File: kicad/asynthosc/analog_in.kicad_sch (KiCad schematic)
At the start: 18 parts, among them J2 AudioJack2, J5 AudioJack2, Q1 Q_NPN_BEC, SW1 TRG0, SW2 ${SIM.PARAMS}, U3 MCP6004

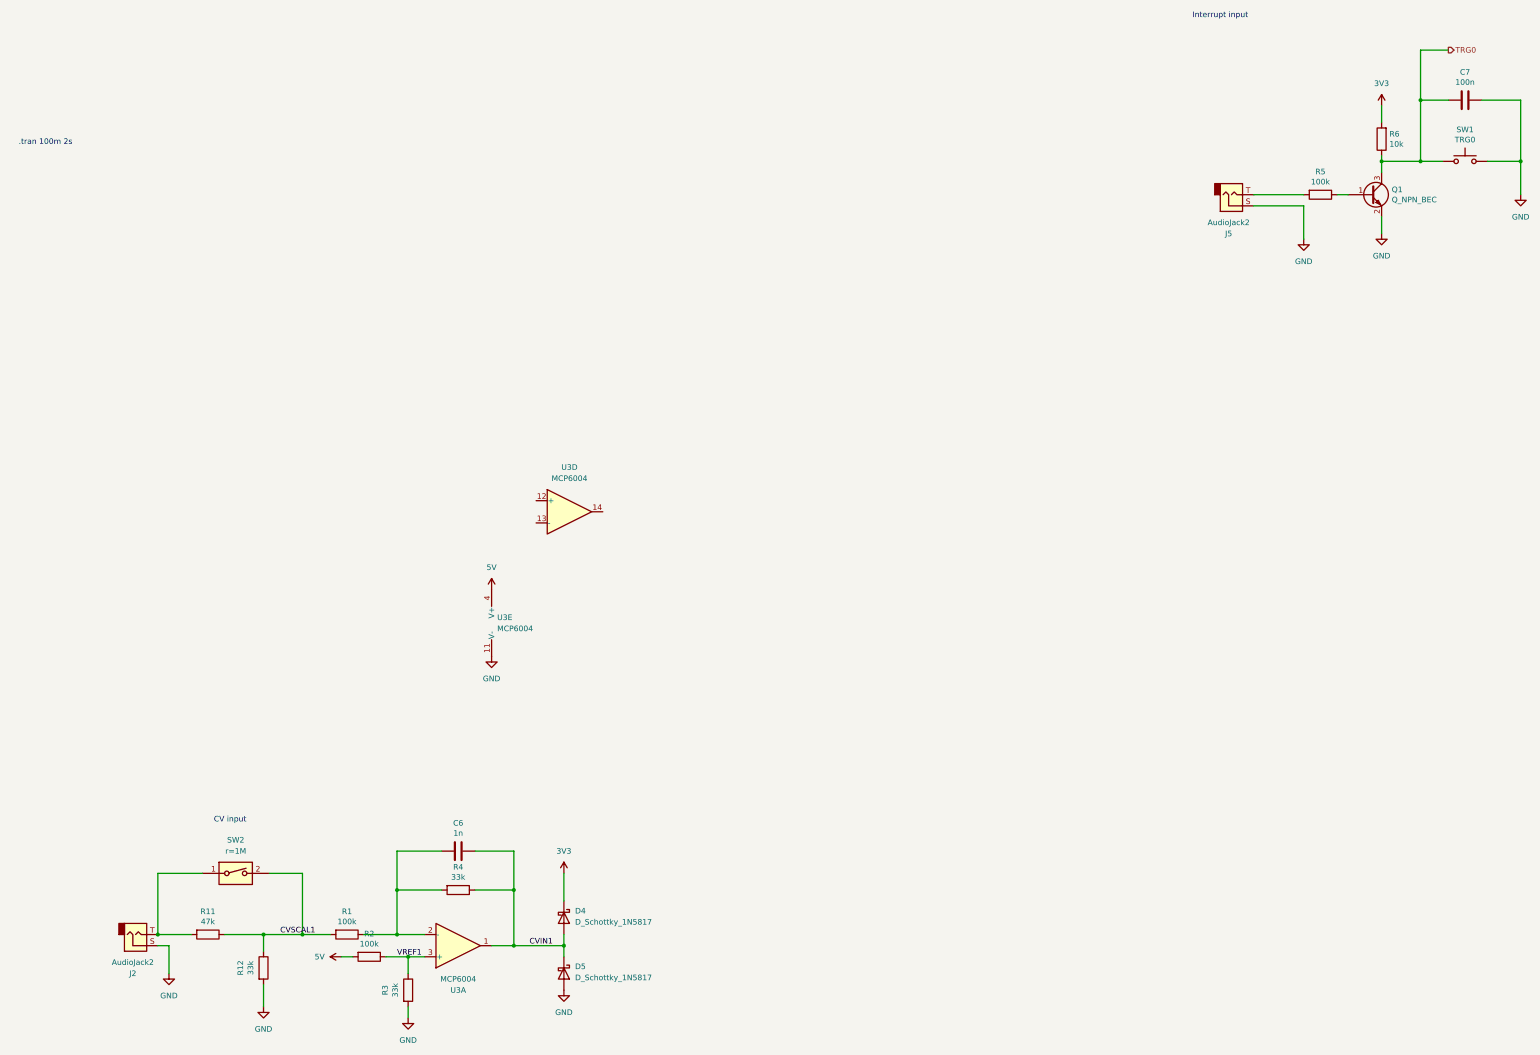
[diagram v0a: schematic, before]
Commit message: sch: wip
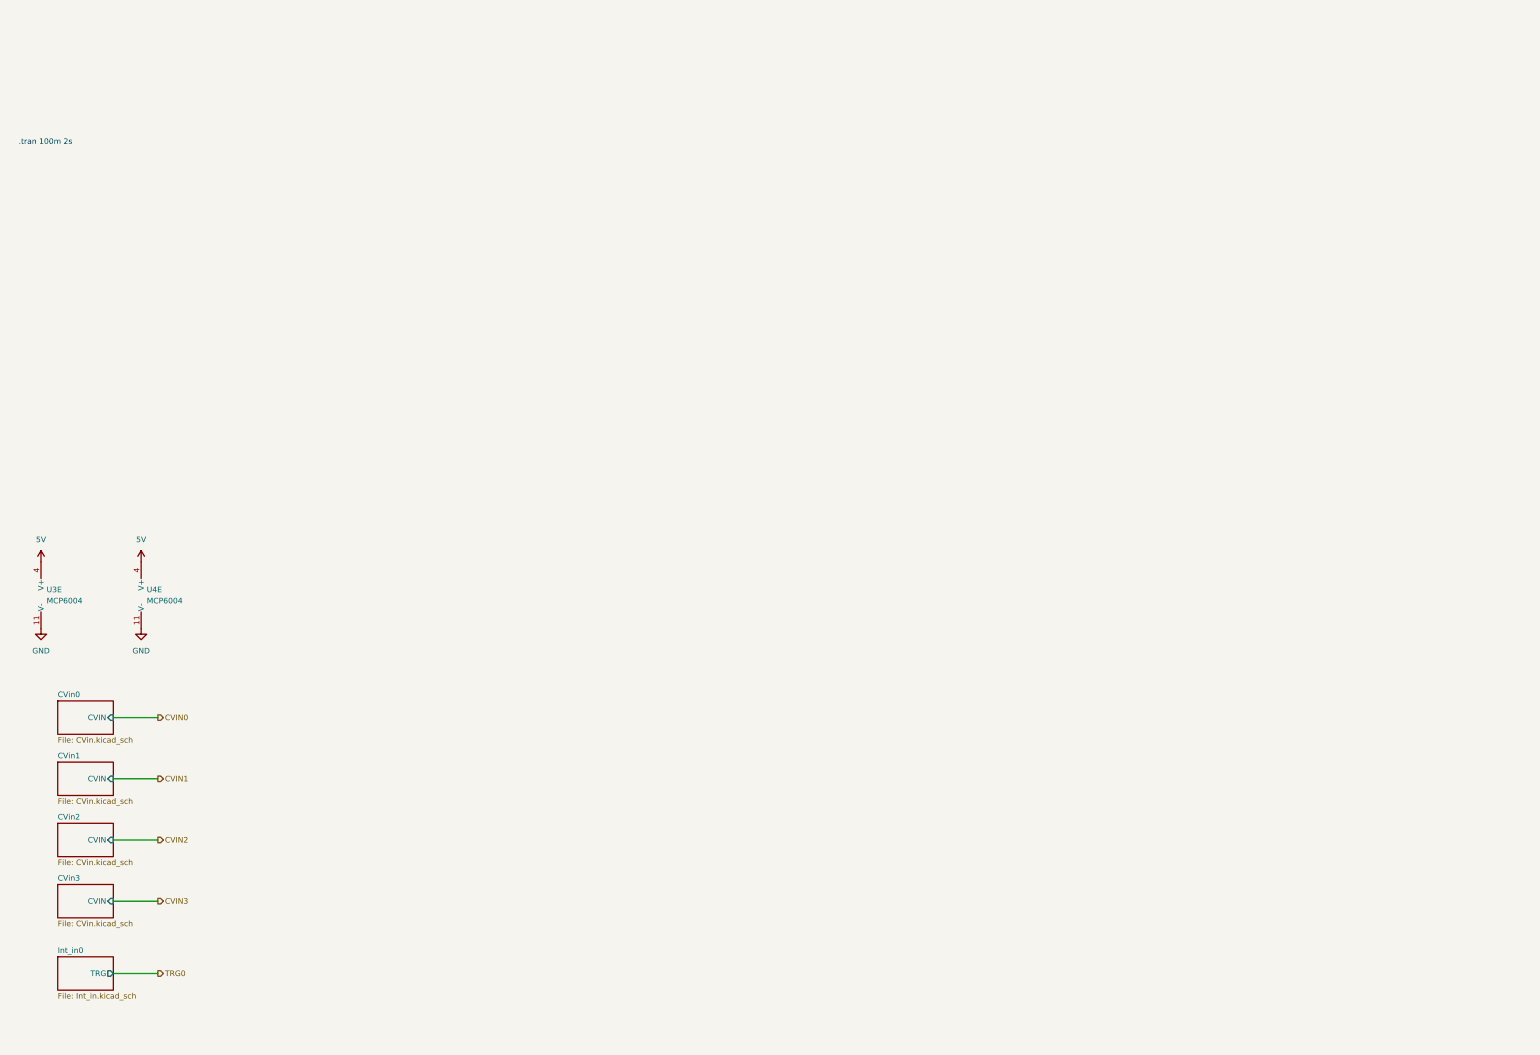
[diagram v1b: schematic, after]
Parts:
- removed C6: 1n, Capacitor_SMD:C_0603_1608Metric, symbol Device:C
- removed C7: 100n, Capacitor_SMD:C_0603_1608Metric, symbol Device:C
- removed D4, D5: D_Schottky_1N5817, symbol Device:D_Schottky
- removed J2, J5: AudioJack2, symbol Connector_Audio:AudioJack2
- removed Q1: Q_NPN_BEC, Package_TO_SOT_SMD:SOT-23, symbol Device:Q_NPN_BEC
- removed R1, R2, R5: 100k, Resistor_SMD:R_0603_1608Metric, symbol Device:R
- removed R11: 47k, Resistor_SMD:R_0603_1608Metric, symbol Device:R
- removed R12, R3, R4: 33k, Resistor_SMD:R_0603_1608Metric, symbol Device:R
- removed R6: 10k, Resistor_SMD:R_0603_1608Metric, symbol Device:R
- removed SW1: TRG0, switches:SW_6425, symbol Switch:SW_Push
- removed SW2: ${SIM.PARAMS}, symbol Switch:SW_DIP_x01
- removed unit 4 of U3
- removed unit 1 of U3
- added U3: MCP6004, symbol Amplifier_Operational:MCP6004
- renumbered U3 to U4
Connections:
- net 5V: now also U3.4 (V+)
- net GND: now also U3.11 (V-)
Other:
- added sheet CVin0 (CVin.kicad_sch)
- added sheet CVin1 (CVin.kicad_sch)
- added sheet CVin2 (CVin.kicad_sch)
- added sheet CVin3 (CVin.kicad_sch)
- added sheet Int_in0 (Int_in.kicad_sch)
- note removed: "CV input"
- note removed: "Interrupt input"
- moved on the sheet: U4E
